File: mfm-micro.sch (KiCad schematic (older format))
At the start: 66 parts, among them J1 USB_B_Mini, J2 JST PH 3, J4 SWD_connector, J8 UART_Connector, P1 Peripheral1_connector, P2 Peripheral2_connector, Q1 AO3401A, SW1 SW_DPDT_x2, SW2 PWR_LED_Switch, SW3 STAT_LED_Switch, SW4 SW_RST, U1 USBLC6-2P6, U2 TP4056, U3 XC6206P332MR, U4 STM32L072CBTx

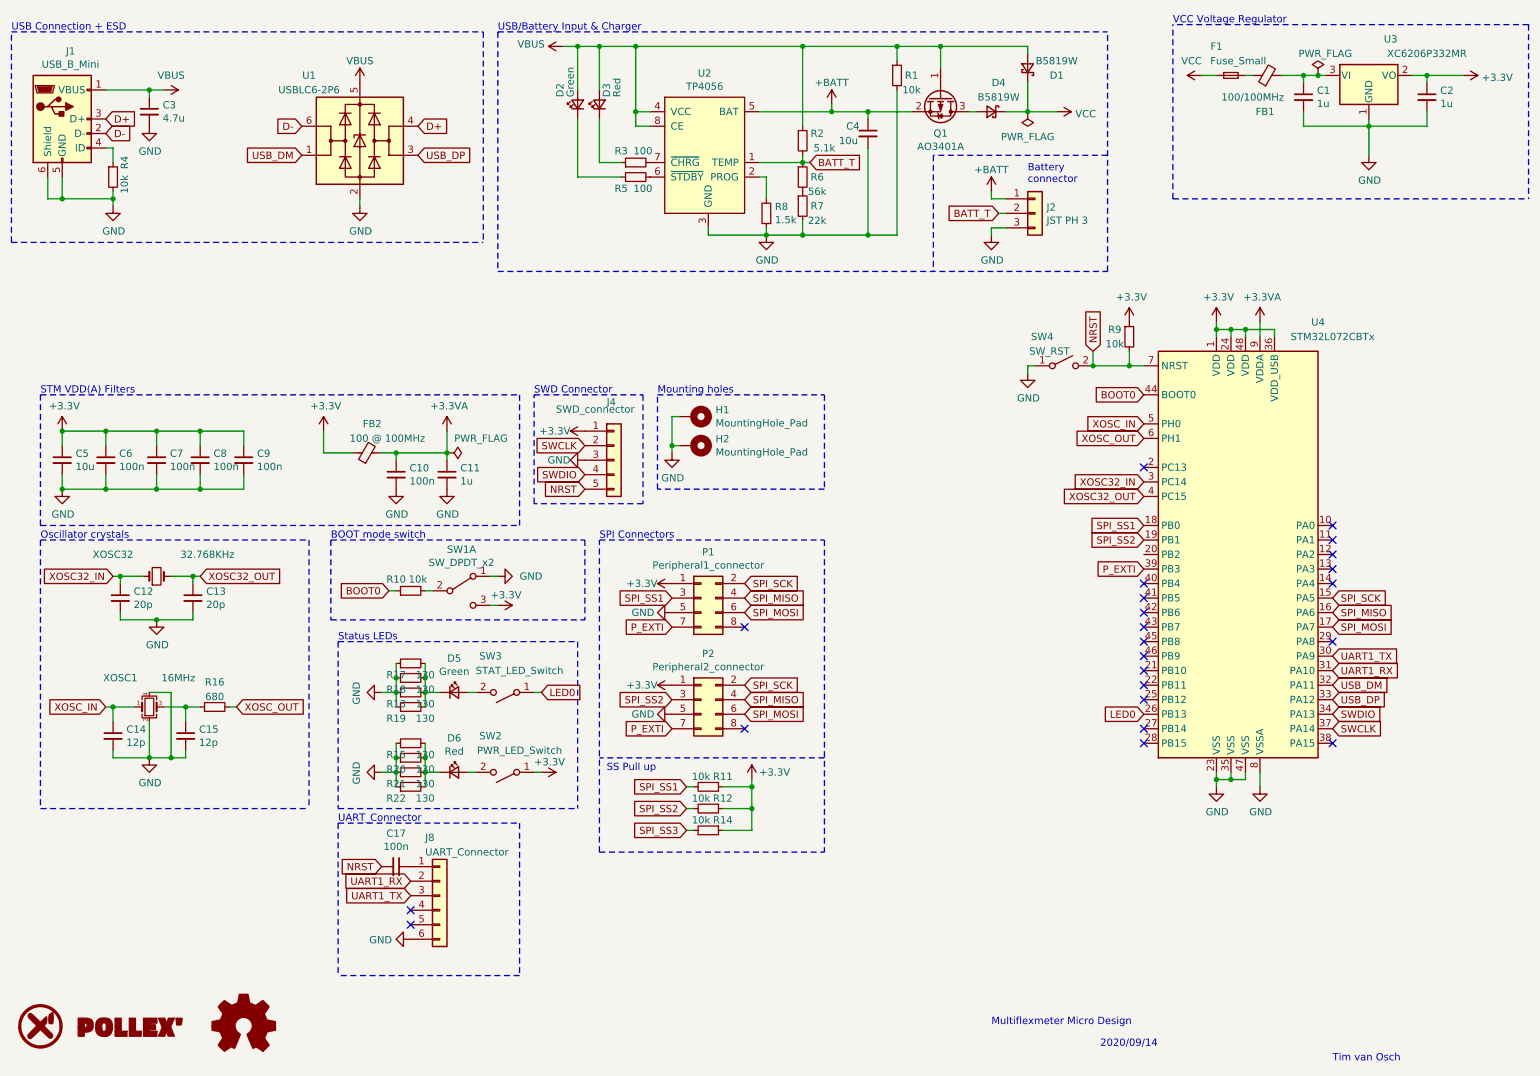
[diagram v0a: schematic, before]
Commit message: Rerout and new exports
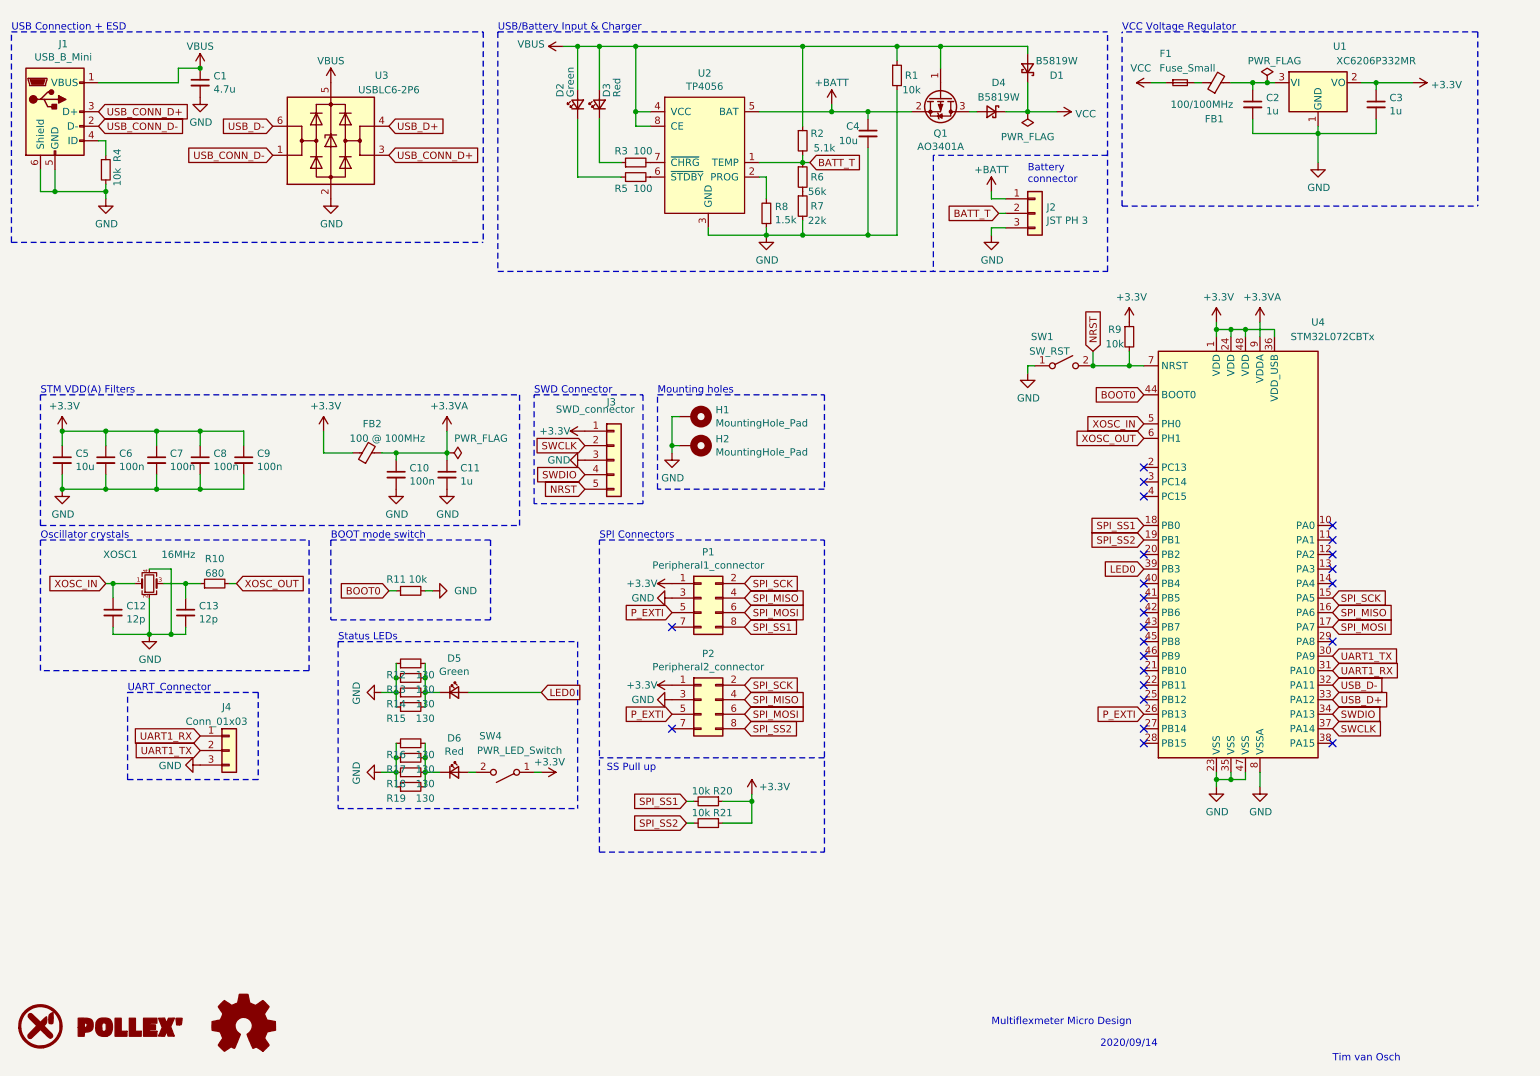
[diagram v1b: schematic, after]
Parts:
- removed C12, C13: 20p, Capacitor_SMD:C_0402_1005Metric, symbol Device:C_Small
- removed C17: 100n, Capacitor_SMD:C_0402_1005Metric, symbol Device:C_Small
- removed J8: UART_Connector, Connector_PinHeader_2.54mm:PinHeader_1x06_P2.54mm_Vertical, symbol Connector_Generic:Conn_01x06
- removed R14: 10k, Resistor_SMD:R_0402_1005Metric, symbol Device:R_Small
- removed SW1: SW_DPDT_x2, Connector_PinHeader_2.54mm:PinHeader_1x03_P2.54mm_Vertical, symbol Switch:SW_DPDT_x2
- removed SW3: STAT_LED_Switch, Connector_PinHeader_2.54mm:PinHeader_1x02_P2.54mm_Vertical, symbol Switch:SW_SPST
- removed XOSC32: 32.768KHz, Crystal:Crystal_SMD_3215-2Pin_3.2x1.5mm, symbol Device:Crystal_Small
- added J4: Conn_01x03, Connector_PinHeader_2.54mm:PinHeader_1x03_P2.54mm_Vertical, symbol Connector_Generic:Conn_01x03
- renumbered C3 to C1, C14 to C12, C15 to C13, C1 to C2, C2 to C3, J4 to J3, R16 to R10, R10 to R11, R17 to R12, R18 to R13, R13 to R14, R19 to R15, R15 to R16, R20 to R17, R21 to R18, R22 to R19, R11 to R20, R12 to R21, SW4 to SW1, SW2 to SW4, U3 to U1, U1 to U3
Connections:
- net GND: now also P1.3 (Pin_3), P2.3 (Pin_3), R11.2, J4.3 (Pin_3); no longer P1.5 (Pin_5), P2.5 (Pin_5)
- net LED0: now also D5.2 (A), U4.39 (PB3); no longer U4.26 (PB13)
- net P_EXTI: now also P1.5 (Pin_5), P2.5 (Pin_5), U4.26 (PB13); no longer P1.7 (Pin_7), P2.7 (Pin_7), U4.39 (PB3)
- net SPI_SS1: now also P1.8 (Pin_8); no longer P1.3 (Pin_3)
- net SPI_SS2: now also P2.8 (Pin_8); no longer P2.3 (Pin_3)
- net UART1_RX: now also J4.1 (Pin_1)
- net UART1_TX: now also J4.2 (Pin_2)
- net D+ renamed USB_CONN_D+
- net USB_CONN_D+: now also U3.3 (I/O2); no longer U3.4 (I/O2)
- net D- renamed USB_CONN_D-
- net USB_CONN_D-: now also U3.1 (I/O1); no longer U3.6 (I/O1)
- net USB_DM renamed USB_D-
- net USB_D-: now also U3.6 (I/O1); no longer U3.1 (I/O1)
- net USB_DP renamed USB_D+
- net USB_D+: now also U3.4 (I/O2); no longer U3.3 (I/O2)
- net XOSC32_IN: no longer names the net of U4.3 (PC14)
- net XOSC32_OUT: no longer names the net of U4.4 (PC15)
- no-connect marks 23 -> 24
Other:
- moved on the sheet: C1, C12, C13, C2, C3, F1, FB1, J1, R10, R20, R21, R4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
